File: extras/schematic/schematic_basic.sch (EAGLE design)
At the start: 1 part

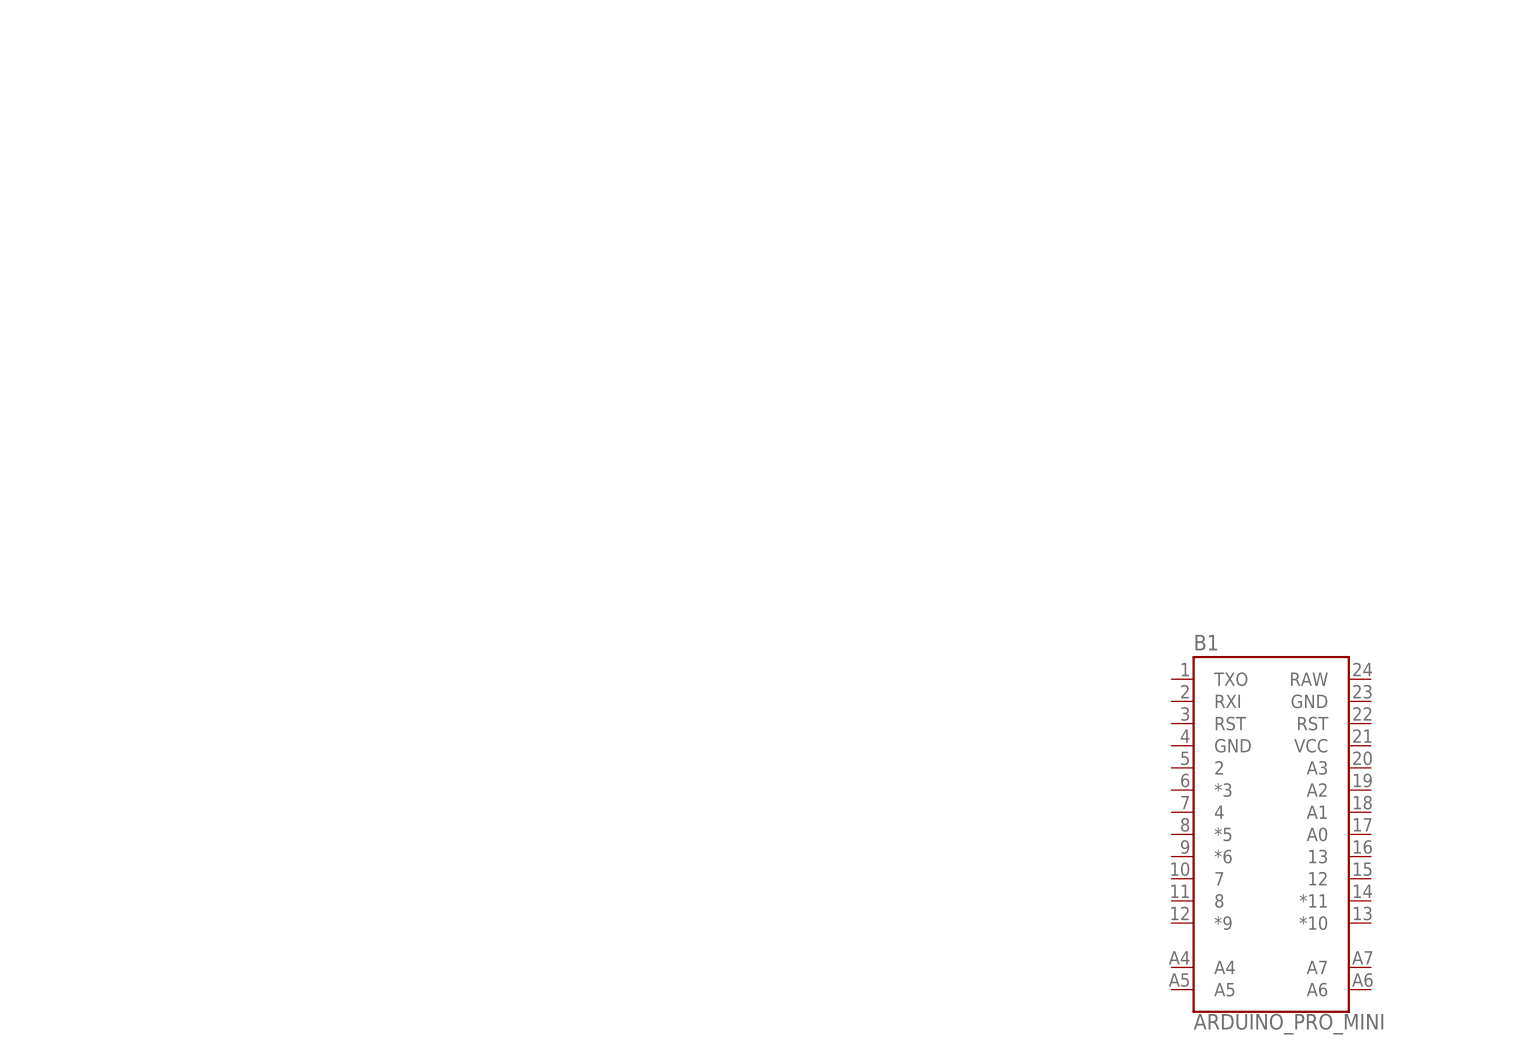
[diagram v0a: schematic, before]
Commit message: SI47XX Arduino LIbrary
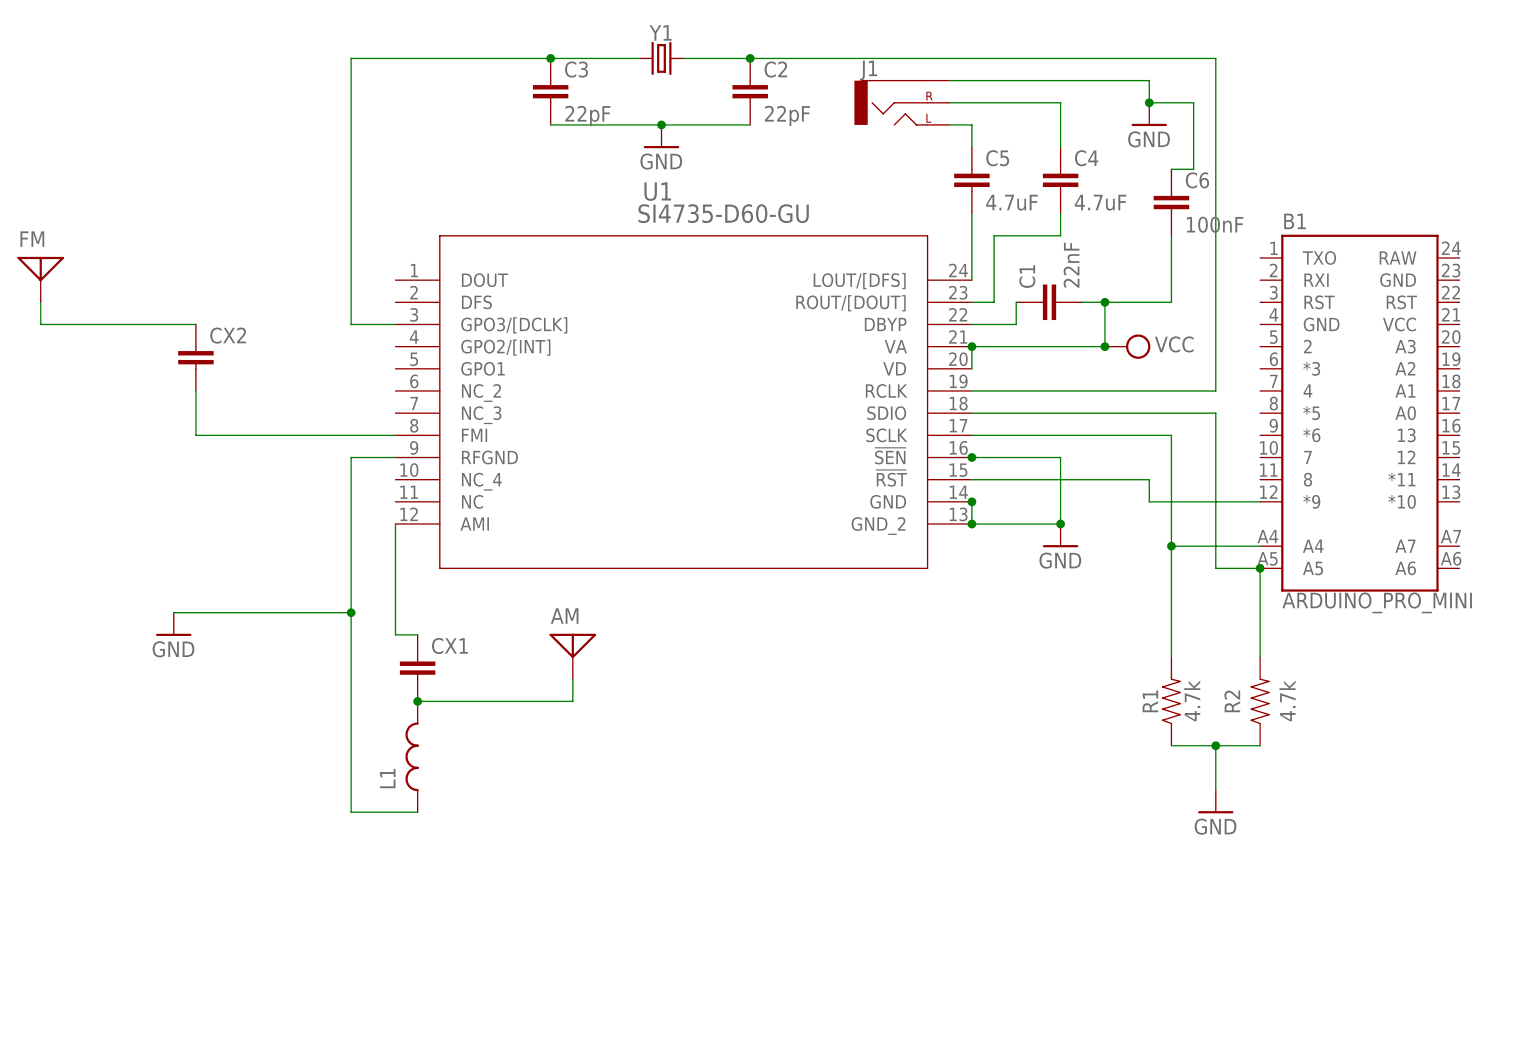
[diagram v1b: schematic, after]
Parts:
- added AM, FM: (no value), discrete:ANTENNA
- added C1: 22nF, SparkFun-Capacitors:22NF/22,000PF-0603-50V-10%
- added C2, C3: 22pF, SparkFun-Capacitors:22PF-0603-50V-5%
- added C4, C5: 4.7uF, SparkFun-Capacitors:4.7UF-1206-16V-(+80/-20%)
- added C6: 100nF, rcl:CXXC10B6
- added CX1, CX2: (no value), rcl:CXXC10B6
- added J1: (no value), SparkFun-Connectors:AUDIO_JACK_2.5MMSPECIAL_POGO_PINS
- added L1: (no value), ngspice-simulation:L
- added R1, R2: 4.7k, SparkFun-Resistors:4.7KOHM-0603-1/10W-1%
- added U1: SI4735-D60-GU, si4735:SI4735-D60-GU
- added Y1: (no value), SparkFun-Clocks:CRYSTALPTH-2X6
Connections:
- new net GND: C2.2, C3.2, C6.1, J1.SLEEVE, L1.1, R1.1, R2.1, U1.!SEN, U1.GND, U1.GND_2, U1.RFGND
- new net N$1: B1.*9, U1.!RST
- new net N$10: AM.1, CX1.2, L1.2
- new net N$12: CX1.1, U1.AMI
- new net N$13: CX2.2, U1.FMI
- new net N$14: CX2.1, FM.1
- new net N$2: B1.A4, R1.2, U1.SCLK
- new net N$3: C2.1, U1.RCLK, Y1.2
- new net N$4: C1.1, U1.DBYP
- new net N$5: C3.1, U1.GPO3/[DCLK], Y1.1
- new net N$6: C5.2, U1.LOUT/[DFS]
- new net N$7: C4.2, U1.ROUT/[DOUT]
- new net N$8: C5.1, J1.LEFT
- new net N$9: C4.1, J1.RIGHT
- new net SDA: B1.A5, R2.2, U1.SDIO
- new net VCC: C1.2, C6.2, U1.VA, U1.VD
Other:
- moved on the sheet: B1
